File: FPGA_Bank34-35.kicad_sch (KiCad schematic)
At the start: 8 parts, among them U8 XC7A35T-FGG484

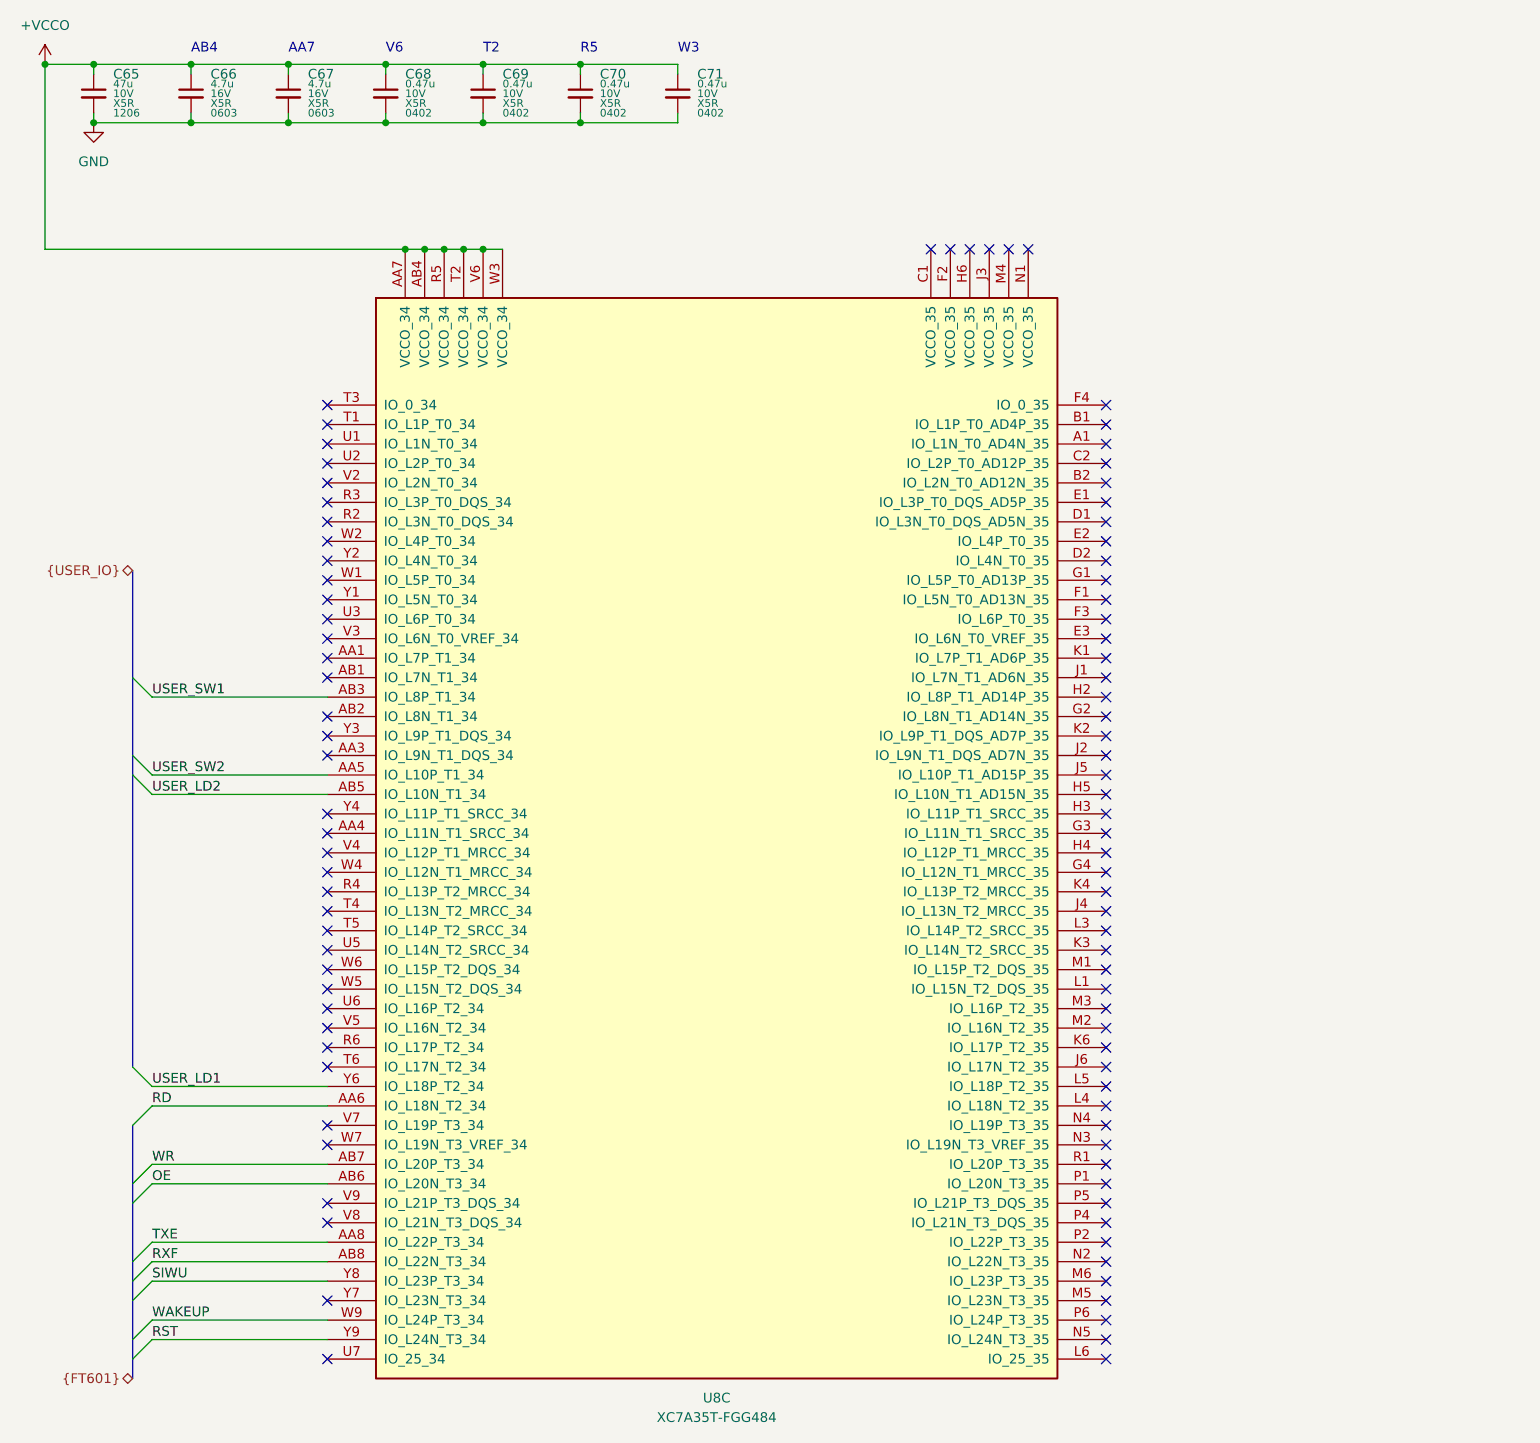
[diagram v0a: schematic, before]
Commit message: Second pass
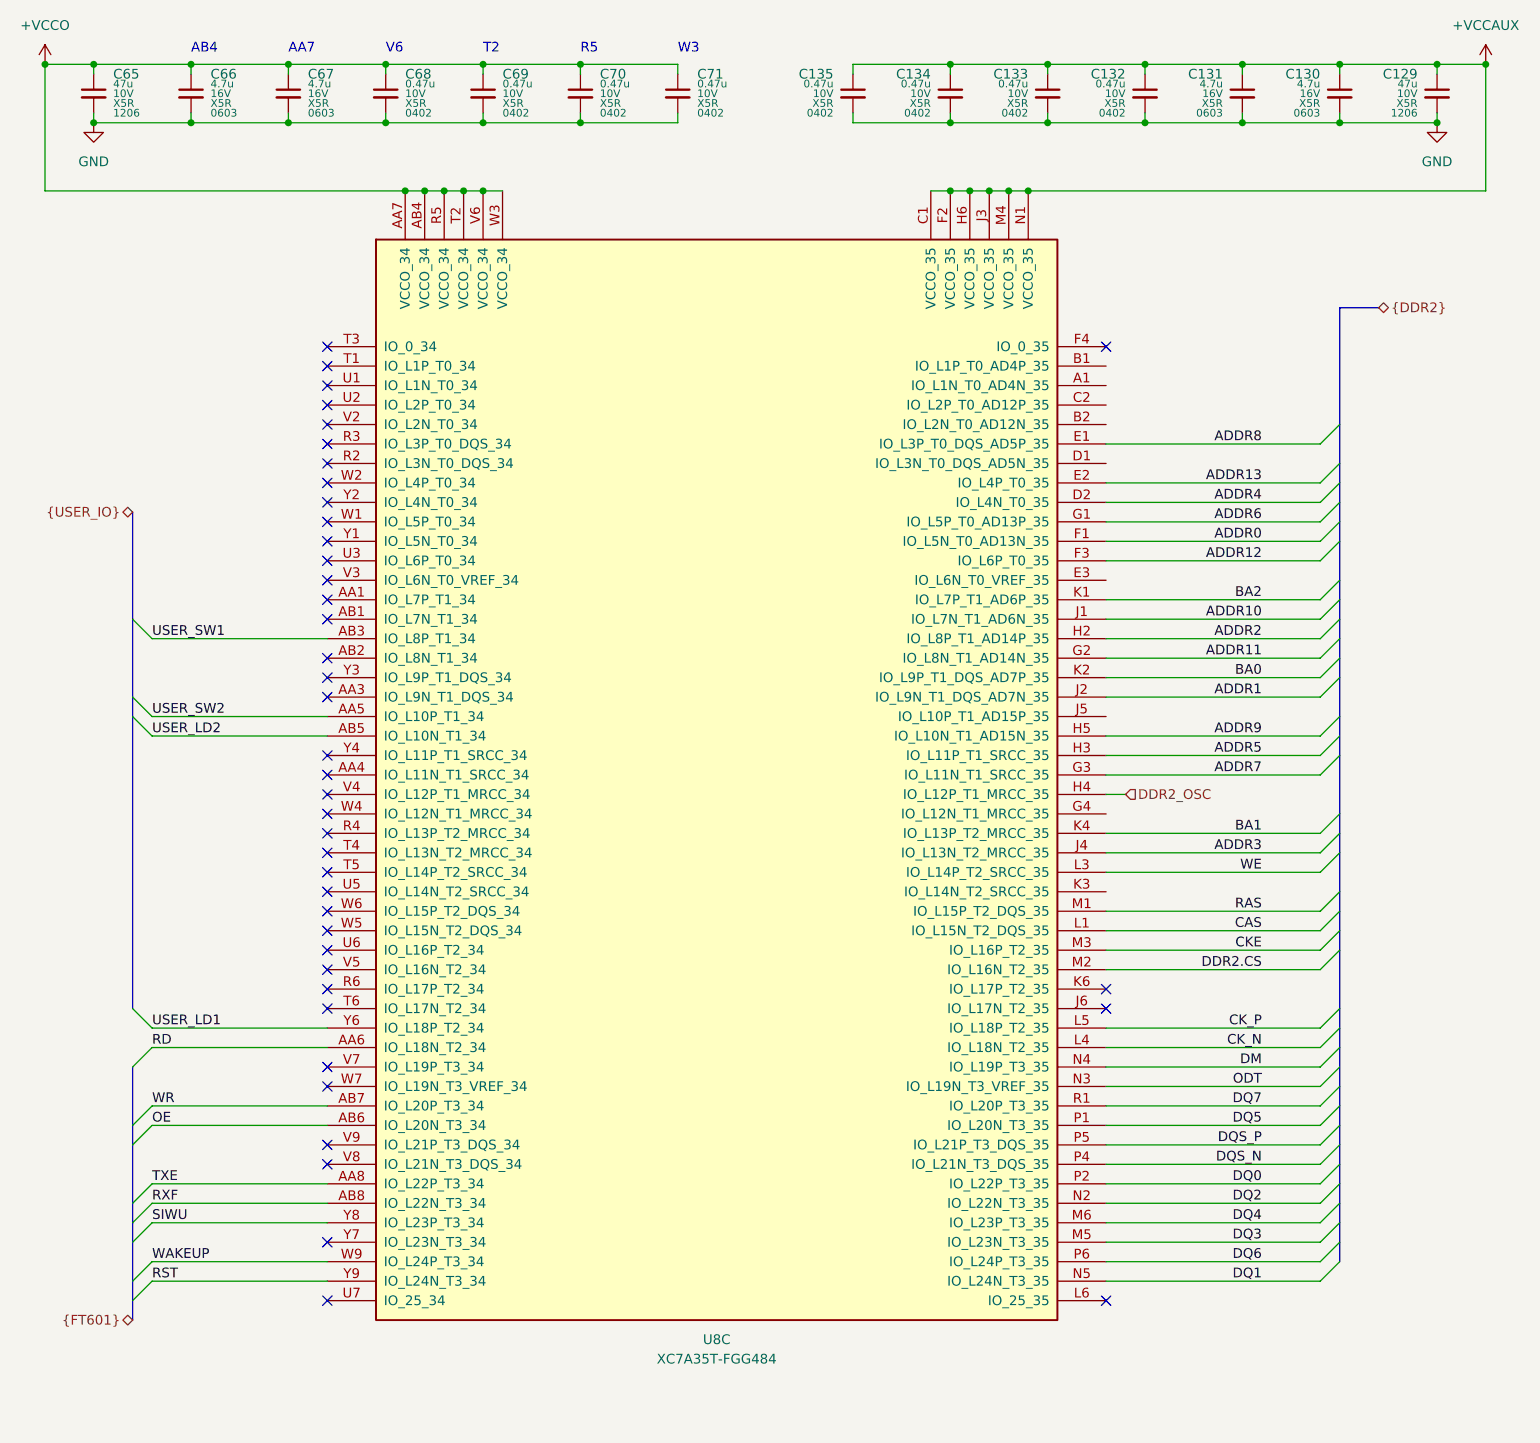
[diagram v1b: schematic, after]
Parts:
- added C129: 47u, Capacitor_SMD:C_1206_3216Metric, symbol Device:C_Small
- added C130, C131: 4.7u, Capacitor_SMD:C_0603_1608Metric, symbol Device:C_Small
- added C132, C133, C134, C135: 0.47u, Capacitor_SMD:C_0402_1005Metric, symbol Device:C_Small
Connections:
- net GND: now also C129.2, C130.2, C131.2, C132.2, C133.2, C134.2, C135.2
- net +VCCAUX: now reaches U8.C1 (VCCO_35)
- net +VCCAUX: now also U8.F2 (VCCO_35), U8.H6 (VCCO_35), U8.J3 (VCCO_35), U8.M4 (VCCO_35), U8.N1 (VCCO_35), C129.1, C130.1, C131.1, C132.1, C133.1, C134.1, C135.1
- net ADDR4: now reaches U8.D2 (IO_L4N_T0_35)
- net ADDR8: now reaches U8.E1 (IO_L3P_T0_DQS_AD5P_35)
- net ADDR13: now reaches U8.E2 (IO_L4P_T0_35)
- net ADDR0: now reaches U8.F1 (IO_L5N_T0_AD13N_35)
- net ADDR12: now reaches U8.F3 (IO_L6P_T0_35)
- net ADDR6: now reaches U8.G1 (IO_L5P_T0_AD13P_35)
- net ADDR11: now reaches U8.G2 (IO_L8N_T1_AD14N_35)
- net ADDR7: now reaches U8.G3 (IO_L11N_T1_SRCC_35)
- net ADDR2: now reaches U8.H2 (IO_L8P_T1_AD14P_35)
- net ADDR5: now reaches U8.H3 (IO_L11P_T1_SRCC_35)
- net DDR2_OSC: now reaches U8.H4 (IO_L12P_T1_MRCC_35)
- net ADDR9: now reaches U8.H5 (IO_L10N_T1_AD15N_35)
- net ADDR10: now reaches U8.J1 (IO_L7N_T1_AD6N_35)
- net ADDR1: now reaches U8.J2 (IO_L9N_T1_DQS_AD7N_35)
- net ADDR3: now reaches U8.J4 (IO_L13N_T2_MRCC_35)
- net BA2: now reaches U8.K1 (IO_L7P_T1_AD6P_35)
- net BA0: now reaches U8.K2 (IO_L9P_T1_DQS_AD7P_35)
- net BA1: now reaches U8.K4 (IO_L13P_T2_MRCC_35)
- net CAS: now reaches U8.L1 (IO_L15N_T2_DQS_35)
- net WE: now reaches U8.L3 (IO_L14P_T2_SRCC_35)
- net CK_N: now reaches U8.L4 (IO_L18N_T2_35)
- net CK_P: now reaches U8.L5 (IO_L18P_T2_35)
- net RAS: now reaches U8.M1 (IO_L15P_T2_DQS_35)
- net DDR2.CS: now reaches U8.M2 (IO_L16N_T2_35)
- net CKE: now reaches U8.M3 (IO_L16P_T2_35)
- net DQ3: now reaches U8.M5 (IO_L23N_T3_35)
- net DQ4: now reaches U8.M6 (IO_L23P_T3_35)
- net DQ2: now reaches U8.N2 (IO_L22N_T3_35)
- net ODT: now reaches U8.N3 (IO_L19N_T3_VREF_35)
- net DM: now reaches U8.N4 (IO_L19P_T3_35)
- net DQ1: now reaches U8.N5 (IO_L24N_T3_35)
- net DQ5: now reaches U8.P1 (IO_L20N_T3_35)
- net DQ0: now reaches U8.P2 (IO_L22P_T3_35)
- net DQS_N: now reaches U8.P4 (IO_L21N_T3_DQS_35)
- net DQS_P: now reaches U8.P5 (IO_L21P_T3_DQS_35)
- net DQ6: now reaches U8.P6 (IO_L24P_T3_35)
- net DQ7: now reaches U8.R1 (IO_L20P_T3_35)
- no-connect marks 94 -> 42
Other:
- moved on the sheet: U8C
